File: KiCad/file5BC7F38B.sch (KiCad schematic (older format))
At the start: 57 parts, among them J301 DB9_Female, P301 ISP/PDI, P302 Thru, P304 Header, SW301 Sync, U301 DS3231, U302 ATmega1284P-AU, U304 SI5351A, U305 74HC1G08, U306 MIC5219-3.3BM5, U307 SN74CB3Q3305, U308 MIC5219-3.3BM5, X301 ASTX-H11-25.MHZ, Y301 20 MHz

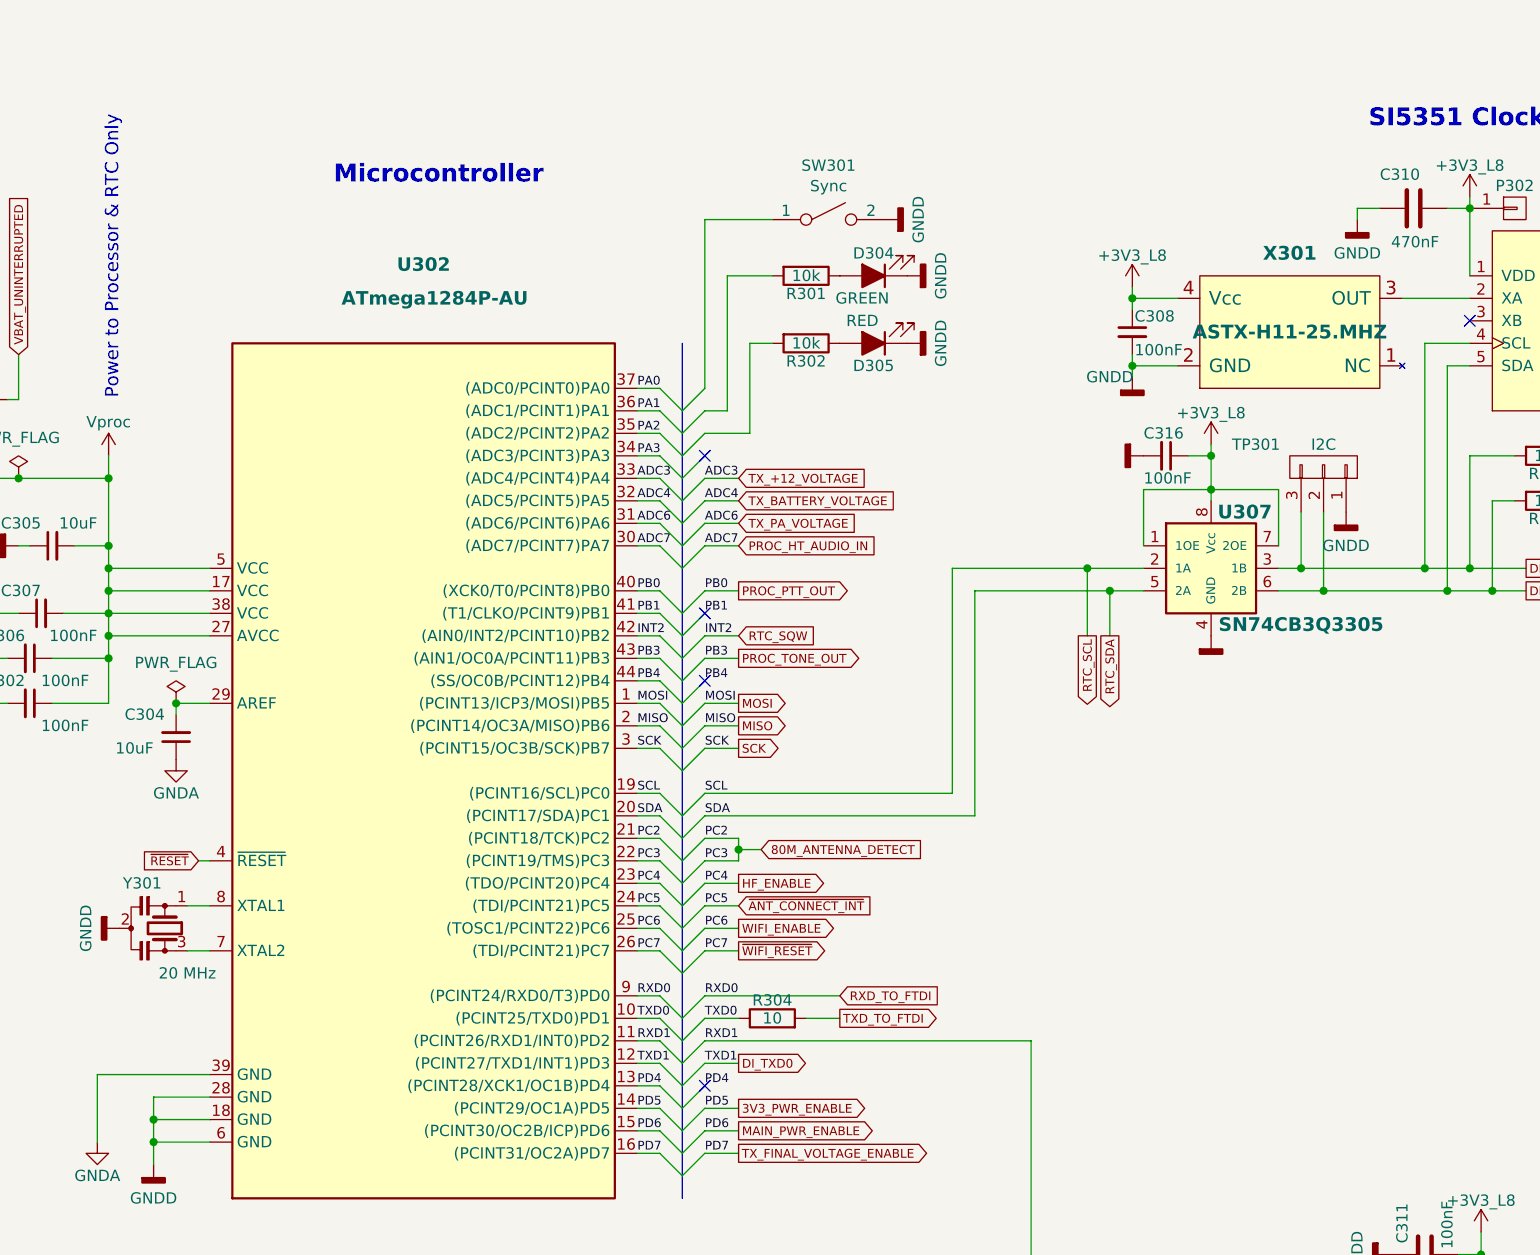
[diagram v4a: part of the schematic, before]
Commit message: Schematic
Schematic changes
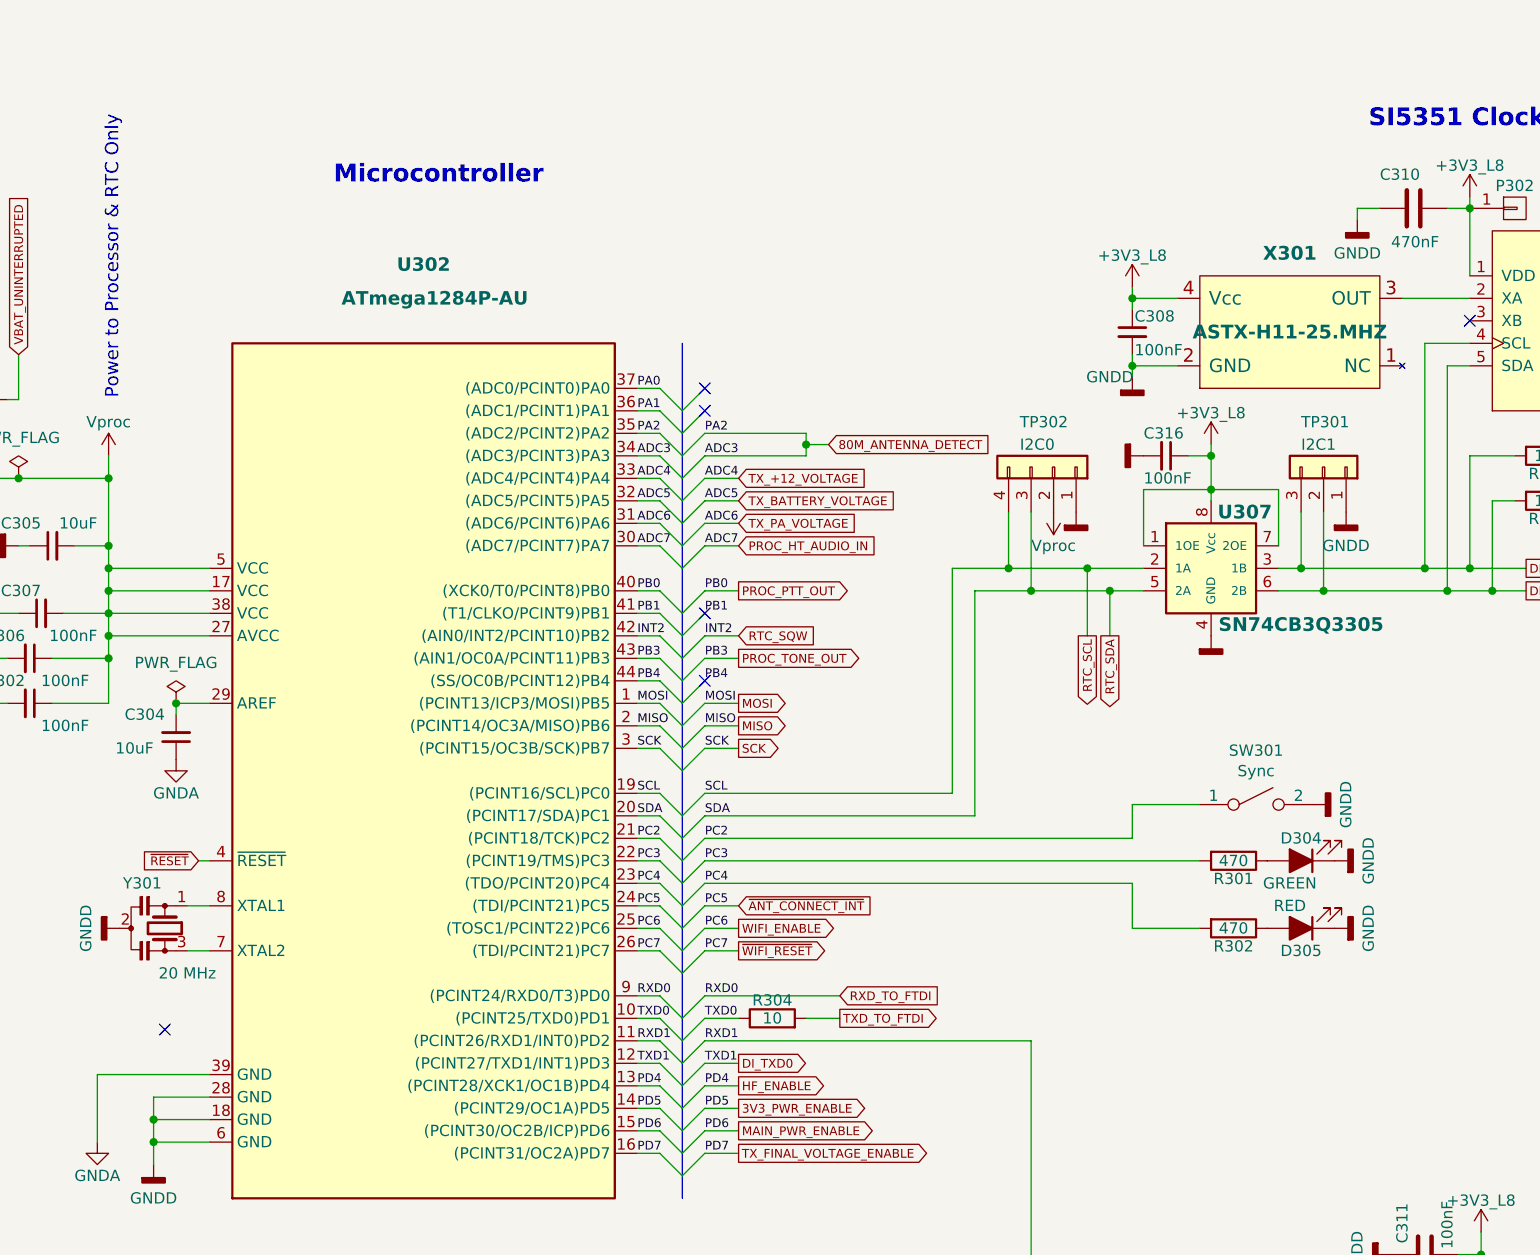
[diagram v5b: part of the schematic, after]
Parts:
- removed TP301: I2C, Pin_Headers:Pin_Header_Straight_1x03, symbol FlexFox80-rescue:CONN_01X03-ARDF-2-Band-MiniTx-rescue
- added TP301: I2C1, symbol Connector_Generic:Conn_01x03
- added TP302: I2C0, symbol Connector_Generic:Conn_01x04
- R301, R302: value 10k -> 470
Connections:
- net PA2 is gone; now on net 80M_ANTENNA_DETECT: U302.35 ((ADC2/PCINT2)PA2)
- net PA3 is gone; now on net 80M_ANTENNA_DETECT: U302.34 ((ADC3/PCINT3)PA3)
- net PD4 is gone; now on net HF_ENABLE: U302.13 ((PCINT28/XCK1/OC1B)PD4)
- net 80M_ANTENNA_DETECT: no longer U302.21 ((PCINT18/TCK)PC2), U302.22 ((PCINT19/TMS)PC3)
- net DI_SCL: now also TP301.3 (Pin_3)
- net DI_SDA: now also TP301.2 (Pin_2)
- net GND: now also TP301.1 (Pin_1), TP302.1 (Pin_1)
- net HF_ENABLE: no longer U302.23 ((TDO/PCINT20)PC4)
- net RTC_SCL: now also TP302.4 (Pin_4)
- net RTC_SDA: now also TP302.3 (Pin_3)
- net Vproc: now also TP302.2 (Pin_2)
- net PC2: now reaches SW301.1
- net PC2: now also U302.21 ((PCINT18/TCK)PC2)
- net PC3: now reaches R301.2
- net PC3: now also U302.22 ((PCINT19/TMS)PC3)
- net PC4: now reaches R302.2
- net PC4: now also U302.23 ((TDO/PCINT20)PC4)
- no-connect marks 15 -> 16
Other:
- moved on the sheet: D304, D305, R301, R302, SW301
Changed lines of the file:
@@
 Wire Wire Line
 	11550 9850 11550 10050
-Wire Wire Line
-	7950 5450 7800 5450
 Text GLabel 7950 3950 2    39   Input ~ 0
 TX_BATTERY_VOLTAGE
 Text GLabel 7950 4050 2    39   Input ~ 0
 TX_PA_VOLTAGE
-Wire Wire Line
-	7950 5550 7800 5550
 Text GLabel 7950 6750 2    39   Output ~ 0
 MAIN_PWR_ENABLE
@@
 Connection ~ 11550 10050
 $Comp
-L FlexFox80-rescue:CONN_01X03-ARDF-2-Band-MiniTx-rescue TP301
-U 1 1 5A0894A0
-P 10550 3800
-F 0 "TP301" V 10650 3500 50  0000 C CNN
-F 1 "I2C" V 10650 3800 50  0000 C CNN
-F 2 "Pin_Headers:Pin_Header_Straight_1x03" H 10550 3800 50  0001 C CNN
-F 3 "" H 10550 3800 50  0001 C CNN
-F 4 "np" H 10550 3800 60  0001 C CNN "Part No."
-F 5 "np" H 10550 3800 60  0001 C CNN "Link"
-	1    10550 3800
-	0    1    -1   0
-$EndComp
-$Comp
 L power:GNDD #PWR0139
 U 1 1 5A0895E4
@@
 Text GLabel 12500 2250 1    39   Output ~ 0
 CLK0
-Text GLabel 7950 5650 2    39   Output ~ 0
+Text GLabel 7950 6550 2    39   Output ~ 0
 HF_ENABLE
 $Comp
@@
 	-1   0    0    1
 $EndComp
-Text GLabel 8050 5500 2    39   Input ~ 0
+Text GLabel 8350 3700 2    39   Input ~ 0
 80M_ANTENNA_DETECT
 Wire Wire Line
-	8050 5500 7950 5500
-Wire Wire Line
-	7950 5450 7950 5500
-Connection ~ 7950 5500
+	8350 3700 8250 3700
+Wire Wire Line
+	8250 3650 8250 3700
+Connection ~ 8250 3700
 Text GLabel 12500 3350 2    39   Output ~ 0
 CLK2
@@
 	13500 7750 13800 7750
 Wire Wire Line
-	7950 5500 7950 5550
+	8250 3700 8250 3750
 Wire Wire Line
 	2450 3500 2750 3500
@@
 	7800 6850 7950 6850
 Wire Wire Line
-	7800 5650 7950 5650
-Wire Wire Line
 	5600 4850 5450 4850
 Connection ~ 5450 4850
@@
 	7950 3850 7800 3850
 Text Label 7500 3950 0    39   ~ 0
-ADC4
+ADC5
 Entry Wire Line
 	7700 6050 7800 5950
 NoConn ~ 7800 4750
 Text Label 7500 3850 0    39   ~ 0
-ADC3
+ADC4
 Text Label 7800 4150 0    39   ~ 0
 ADC7
@@
 ADC6
 Text Label 7800 3950 0    39   ~ 0
+ADC5
+Text Label 7800 3850 0    39   ~ 0
 ADC4
-Text Label 7800 3850 0    39   ~ 0
-ADC3
 Text Label 7800 6150 0    39   ~ 0
 RXD0
@@
 	9000 5350 9000 4350
 Wire Wire Line
-	9000 4350 9600 4350
-Wire Wire Line
-	8900 4250 9500 4250
+	9000 4350 9250 4350
+Wire Wire Line
+	8900 4250 9150 4250
 Wire Wire Line
 	9500 4550 9500 4250
@@
 Text Label 7500 3650 0    39   ~ 0
 PA2
-Text Label 7500 3750 0    39   ~ 0
-PA3
 Text GLabel 7950 4350 2    39   Output ~ 0
 PROC_PTT_OUT
@@
 Wire Wire Line
 	5500 5950 5600 5950
-NoConn ~ 7800 3750
-NoConn ~ 7800 6550
 $Comp
 L Connector:DB9_Female J301
@@
 L Device:LED_ALT D304
 U 1 1 61B9E05F
-P 8550 2950
-F 0 "D304" H 8550 2850 50  0000 C CNN
-F 1 "GREEN" H 8600 3050 50  0000 C CNN
-F 2 "" H 8550 2950 50  0001 C CNN
-F 3 "~" H 8550 2950 50  0001 C CNN
-	1    8550 2950
+P 10450 5550
+F 0 "D304" H 10450 5450 50  0000 C CNN
+F 1 "GREEN" H 10500 5650 50  0000 C CNN
+F 2 "" H 10450 5550 50  0001 C CNN
+F 3 "~" H 10450 5550 50  0001 C CNN
+	1    10450 5550
 	-1   0    0    1
 $EndComp
@@
 L Device:LED_ALT D305
 U 1 1 61BA0B72
-P 8550 3250
-F 0 "D305" H 8550 3350 50  0000 C CNN
-F 1 "RED" H 8600 3150 50  0000 C CNN
-F 2 "" H 8550 3250 50  0001 C CNN
-F 3 "~" H 8550 3250 50  0001 C CNN
-	1    8550 3250
+P 10450 5850
+F 0 "D305" H 10450 5950 50  0000 C CNN
+F 1 "RED" H 10500 5750 50  0000 C CNN
+F 2 "" H 10450 5850 50  0001 C CNN
+F 3 "~" H 10450 5850 50  0001 C CNN
+	1    10450 5850
 	-1   0    0    1
 $EndComp
@@
 L Switch:SPST_small SW301
 U 1 1 61BA254A
-P 8350 2700
-F 0 "SW301" H 8350 2940 50  0000 C CNN
-F 1 "Sync" H 8350 2849 50  0000 C CNN
-F 2 "" H 8350 2700 50  0000 C CNN
-F 3 "" H 8350 2700 50  0000 C CNN
-	1    8350 2700
+P 10250 5300
+F 0 "SW301" H 10250 5540 50  0000 C CNN
+F 1 "Sync" H 10250 5449 50  0000 C CNN
+F 2 "" H 10250 5300 50  0000 C CNN
+F 3 "" H 10250 5300 50  0000 C CNN
+	1    10250 5300
 	1    0    0    -1
 $EndComp
@@
 L Device:R R301
 U 1 1 61C7B255
-P 8250 2950
-F 0 "R301" V 8330 2950 50  0000 C CNN
-F 1 "10k" V 8250 2950 50  0000 C CNN
-F 2 "Resistors_SMD:R_0805_HandSoldering" H 8180 2950 50  0001 C CNN
-F 3 "http://www.yageo.com/documents/recent/PYu-RC_Group_51_RoHS_L_04.pdf" H 8250 2950 50  0001 C CNN
-F 4 "311-10.0KCRCT-ND" H 8250 2950 60  0001 C CNN "Part No."
-F 5 "<a href=\"https://www.digikey.com/products/en?keywords=311-10.0KCRCT-ND\">Link</a>" H 8250 2950 60  0001 C CNN "Link"
-	1    8250 2950
+P 10150 5550
+F 0 "R301" V 10230 5550 50  0000 C CNN
+F 1 "470" V 10150 5550 50  0000 C CNN
+F 2 "Resistors_SMD:R_0805_HandSoldering" H 10080 5550 50  0001 C CNN
+F 3 "http://www.yageo.com/documents/recent/PYu-RC_Group_51_RoHS_L_04.pdf" H 10150 5550 50  0001 C CNN
+F 4 "311-10.0KCRCT-ND" H 10150 5550 60  0001 C CNN "Part No."
+F 5 "<a href=\"https://www.digikey.com/products/en?keywords=311-10.0KCRCT-ND\">Link</a>" H 10150 5550 60  0001 C CNN "Link"
+	1    10150 5550
 	0    1    1    0
 $EndComp
@@
 L Device:R R302
 U 1 1 61C8FCFC
-P 8250 3250
-F 0 "R302" V 8330 3250 50  0000 C CNN
-F 1 "10k" V 8250 3250 50  0000 C CNN
-F 2 "Resistors_SMD:R_0805_HandSoldering" H 8180 3250 50  0001 C CNN
-F 3 "http://www.yageo.com/documents/recent/PYu-RC_Group_51_RoHS_L_04.pdf" H 8250 3250 50  0001 C CNN
-F 4 "311-10.0KCRCT-ND" H 8250 3250 60  0001 C CNN "Part No."
-F 5 "<a href=\"https://www.digikey.com/products/en?keywords=311-10.0KCRCT-ND\">Link</a>" H 8250 3250 60  0001 C CNN "Link"
-	1    8250 3250
+P 10150 5850
+F 0 "R302" V 10230 5850 50  0000 C CNN
+F 1 "470" V 10150 5850 50  0000 C CNN
+F 2 "Resistors_SMD:R_0805_HandSoldering" H 10080 5850 50  0001 C CNN
+F 3 "http://www.yageo.com/documents/recent/PYu-RC_Group_51_RoHS_L_04.pdf" H 10150 5850 50  0001 C CNN
+F 4 "311-10.0KCRCT-ND" H 10150 5850 60  0001 C CNN "Part No."
+F 5 "<a href=\"https://www.digikey.com/products/en?keywords=311-10.0KCRCT-ND\">Link</a>" H 10150 5850 60  0001 C CNN "Link"
+	1    10150 5850
 	0    1    1    0
 $EndComp
@@
 L power:GNDD #PWR?
 U 1 1 61CAFDE2
-P 8600 2700
-F 0 "#PWR?" H 8600 2450 50  0001 C CNN
-F 1 "GNDD" H 8600 2550 50  0000 C CNN
-F 2 "" H 8600 2700 50  0000 C CNN
-F 3 "" H 8600 2700 50  0000 C CNN
-	1    8600 2700
+P 10500 5300
+F 0 "#PWR?" H 10500 5050 50  0001 C CNN
+F 1 "GNDD" H 10500 5150 50  0000 C CNN
+F 2 "" H 10500 5300 50  0000 C CNN
+F 3 "" H 10500 5300 50  0000 C CNN
+	1    10500 5300
 	0    -1   -1   0
 $EndComp
@@
 L power:GNDD #PWR?
 U 1 1 61CB2436
-P 8700 2950
-F 0 "#PWR?" H 8700 2700 50  0001 C CNN
-F 1 "GNDD" H 8700 2800 50  0000 C CNN
-F 2 "" H 8700 2950 50  0000 C CNN
-F 3 "" H 8700 2950 50  0000 C CNN
-	1    8700 2950
+P 10600 5550
+F 0 "#PWR?" H 10600 5300 50  0001 C CNN
+F 1 "GNDD" H 10600 5400 50  0000 C CNN
+F 2 "" H 10600 5550 50  0000 C CNN
+F 3 "" H 10600 5550 50  0000 C CNN
+	1    10600 5550
 	0    -1   -1   0
 $EndComp
@@
 L power:GNDD #PWR?
 U 1 1 61CB3557
-P 8700 3250
-F 0 "#PWR?" H 8700 3000 50  0001 C CNN
-F 1 "GNDD" H 8700 3100 50  0000 C CNN
-F 2 "" H 8700 3250 50  0000 C CNN
-F 3 "" H 8700 3250 50  0000 C CNN
-	1    8700 3250
+P 10600 5850
+F 0 "#PWR?" H 10600 5600 50  0001 C CNN
+F 1 "GNDD" H 10600 5700 50  0000 C CNN
+F 2 "" H 10600 5850 50  0000 C CNN
+F 3 "" H 10600 5850 50  0000 C CNN
+	1    10600 5850
 	0    -1   -1   0
 $EndComp
 Wire Wire Line
-	7800 3450 7800 2700
-Wire Wire Line
-	7800 2700 8100 2700
-Wire Wire Line
-	7800 3550 7900 3550
-Wire Wire Line
-	7900 3550 7900 2950
-Wire Wire Line
-	7900 2950 8100 2950
-Wire Wire Line
-	7800 3650 8000 3650
-Wire Wire Line
-	8000 3650 8000 3250
-Wire Wire Line
-	8000 3250 8100 3250
+	9700 5300 10000 5300
+Wire Wire Line
+	7800 6550 7950 6550
+Wire Wire Line
+	7800 5450 9700 5450
+Wire Wire Line
+	9700 5450 9700 5300
+Wire Wire Line
+	7800 5550 10000 5550
+Wire Wire Line
+	9700 5650 9700 5850
+Wire Wire Line
+	7800 5650 9700 5650
+Wire Wire Line
+	9700 5850 10000 5850
+Wire Wire Line
+	7800 3650 8250 3650
+Wire Wire Line
+	7800 3750 8250 3750
+Text Label 7800 3750 0    39   ~ 0
+ADC3
+Text Label 7500 3750 0    39   ~ 0
+ADC3
+Text Label 7800 3650 0    39   ~ 0
+PA2
+NoConn ~ 7800 3450
+NoConn ~ 7800 3550
+$Comp
+L power:GNDD #PWR?
+U 1 1 60878579
+P 9450 4000
+F 0 "#PWR?" H 9450 3750 50  0001 C CNN
+F 1 "GNDD" H 9600 3850 50  0001 C CNN
+F 2 "" H 9450 4000 50  0000 C CNN
+F 3 "" H 9450 4000 50  0000 C CNN
+	1    9450 4000
+	1    0    0    -1
+$EndComp
+Wire Wire Line
+	9150 4000 9150 4250
+Wire Wire Line
+	9250 4000 9250 4350
+Connection ~ 9150 4250
+Wire Wire Line
+	9150 4250 9500 4250
+Connection ~ 9250 4350
+Wire Wire Line
+	9250 4350 9600 4350
+NoConn ~ 5400 6300
+$Comp
+L FlexFox80-rescue:Vproc-ARDF-2-Band-MiniTx-rescue #PWR?
+U 1 1 608A7865
+P 9350 4000
+F 0 "#PWR?" H 9350 3850 50  0001 C CNN
+F 1 "Vproc" H 9350 4150 50  0000 C CNN
+F 2 "" H 9350 4000 50  0000 C CNN
+F 3 "" H 9350 4000 50  0000 C CNN
+	1    9350 4000
+	-1   0    0    1
+$EndComp
+$Comp
+L Connector_Generic:Conn_01x04 TP302
+U 1 1 608ADA8E
+P 9350 3800
+F 0 "TP302" V 9550 3650 50  0000 L CNN
+F 1 "I2C0" V 9450 3650 50  0000 L CNN
+F 2 "" H 9350 3800 50  0001 C CNN
+F 3 "~" H 9350 3800 50  0001 C CNN
+	1    9350 3800
+	0    1    -1   0
+$EndComp
+$Comp
+L Connector_Generic:Conn_01x03 TP301
+U 1 1 608CC2B9
+P 10550 3800
+F 0 "TP301" V 10750 3700 50  0000 L CNN
+F 1 "I2C1" V 10650 3700 50  0000 L CNN
+F 2 "" H 10550 3800 50  0001 C CNN
+F 3 "~" H 10550 3800 50  0001 C CNN
+	1    10550 3800
+	0    1    -1   0
+$EndComp
 Wire Bus Line
 	7700 3250 7700 7050
